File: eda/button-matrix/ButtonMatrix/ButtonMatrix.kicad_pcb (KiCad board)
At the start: 2 copper layers, 191.5 x 87.2 mm, 18 parts, among them SW1 SW_Omron_B3FS, SW10 SW_Omron_B3FS, SW11 SW_Omron_B3FS, SW12 SW_Omron_B3FS, SW13 SW_Omron_B3FS, SW14 SW_Omron_B3FS, SW15 SW_Omron_B3FS, SW16 SW_Omron_B3FS, SW2 SW_Omron_B3FS, SW3 SW_Omron_B3FS, SW4 SW_Omron_B3FS, SW5 SW_Omron_B3FS, SW6 SW_Omron_B3FS, SW7 SW_Omron_B3FS, SW8 SW_Omron_B3FS, SW9 SW_Omron_B3FS

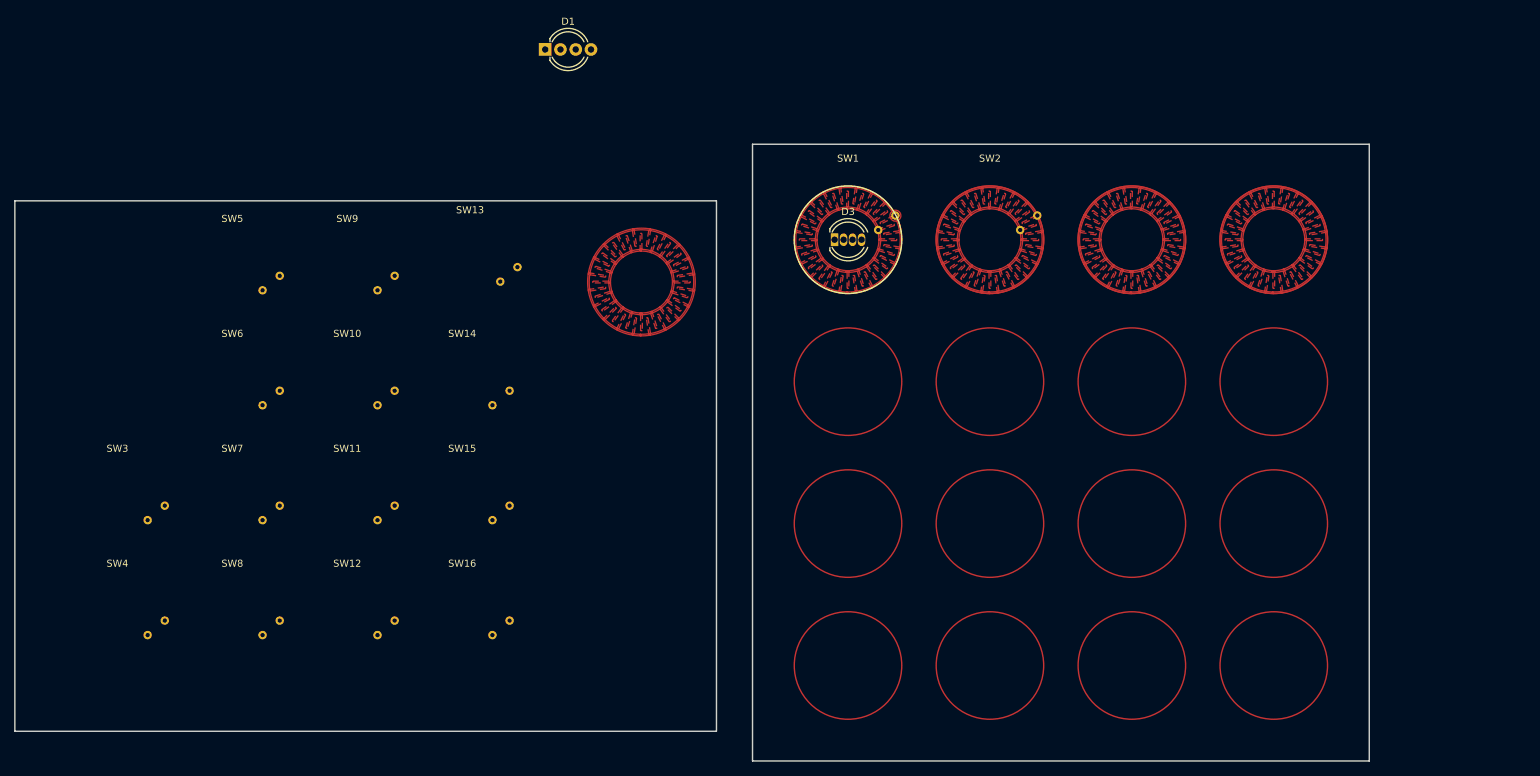
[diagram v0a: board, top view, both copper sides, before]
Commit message: - Updated the pcb for the new 4x4 button matrix - Added support imgui and desktop support
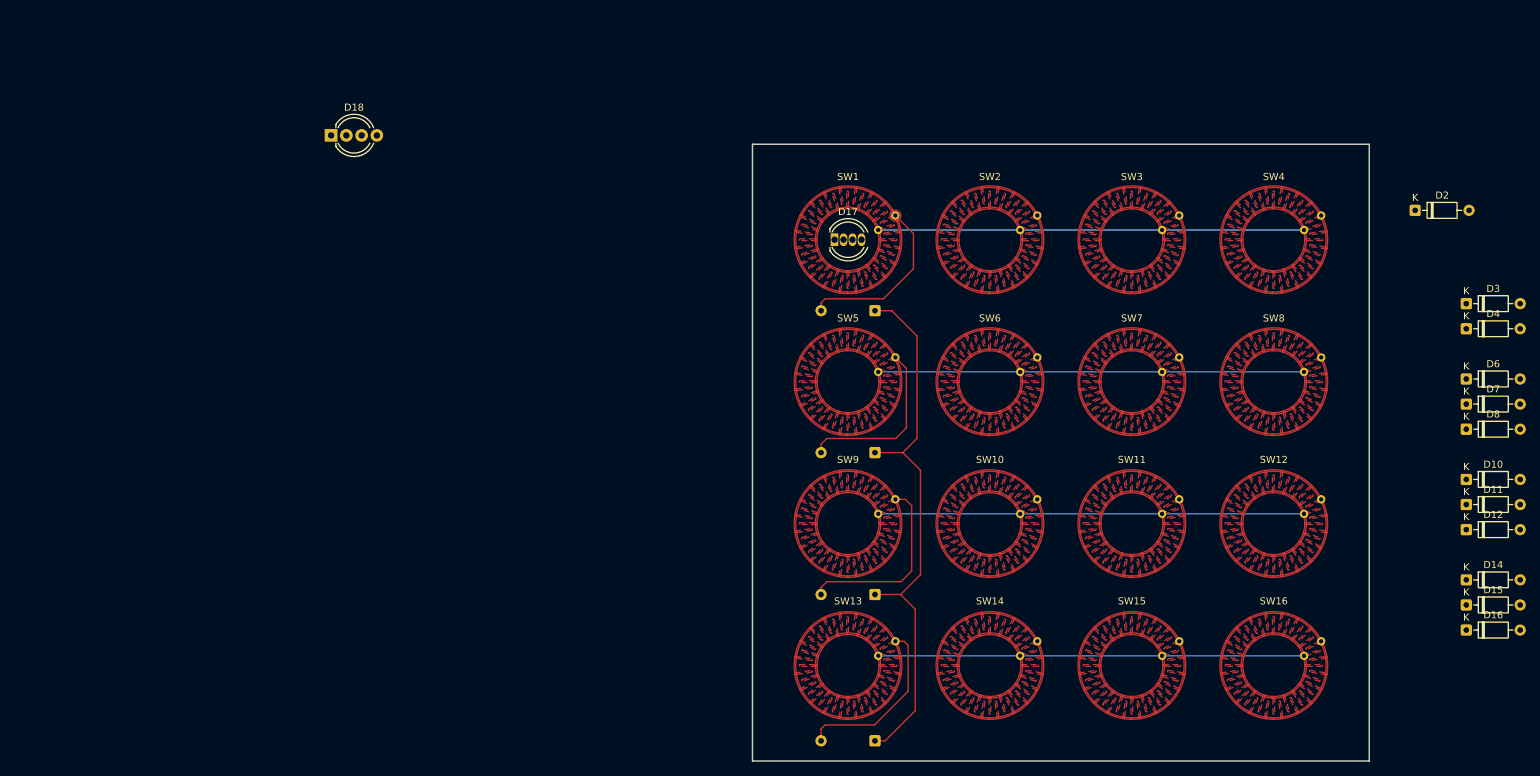
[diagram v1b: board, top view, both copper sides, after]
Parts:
- added D10: 1N4148, Diode_THT:D_DO-35_SOD27_P7.62mm_Horizontal, F.Cu at (228.9, 106.8)
- added D11: 1N4148, Diode_THT:D_DO-35_SOD27_P7.62mm_Horizontal, F.Cu at (228.9, 110.3)
- added D12: 1N4148, Diode_THT:D_DO-35_SOD27_P7.62mm_Horizontal, F.Cu at (228.9, 113.9)
- added D13: 1N4148, Diode_THT:D_DO-35_SOD27_P7.62mm_Horizontal, B.Cu at (145.3, 143.8)
- added D14: 1N4148, Diode_THT:D_DO-35_SOD27_P7.62mm_Horizontal, F.Cu at (228.9, 121.0)
- added D15: 1N4148, Diode_THT:D_DO-35_SOD27_P7.62mm_Horizontal, F.Cu at (228.9, 124.5)
- added D16: 1N4148, Diode_THT:D_DO-35_SOD27_P7.62mm_Horizontal, F.Cu at (228.9, 128.1)
- added D17: LED_RGBA, LED_THT:LED_D5.0mm-4_RGB, F.Cu at (139.6, 72.9)
- added D18: LED_RGBA, LED_THT:LED_D5.0mm-4_RGB_Wide_Pins, F.Cu at (68.4, 58.1)
- added D2: 1N4148, Diode_THT:D_DO-35_SOD27_P7.62mm_Horizontal, F.Cu at (221.7, 68.8)
- added D4: 1N4148, Diode_THT:D_DO-35_SOD27_P7.62mm_Horizontal, F.Cu at (228.9, 85.5)
- added D5: 1N4148, Diode_THT:D_DO-35_SOD27_P7.62mm_Horizontal, B.Cu at (145.3, 103.0)
- added D6: 1N4148, Diode_THT:D_DO-35_SOD27_P7.62mm_Horizontal, F.Cu at (228.9, 92.6)
- added D7: 1N4148, Diode_THT:D_DO-35_SOD27_P7.62mm_Horizontal, F.Cu at (228.9, 96.1)
- added D8: 1N4148, Diode_THT:D_DO-35_SOD27_P7.62mm_Horizontal, F.Cu at (228.9, 99.7)
- added D9: 1N4148, Diode_THT:D_DO-35_SOD27_P7.62mm_Horizontal, B.Cu at (145.3, 123.1)
- D1: value LED_RGBA -> 1N4148; footprint LED_THT:LED_D5.0mm-4_RGB_Wide_Pins -> Diode_THT:D_DO-35_SOD27_P7.62mm_Horizontal; moved to B.Cu
- D3: value LED_RGBA -> 1N4148; footprint LED_THT:LED_D5.0mm-4_RGB -> Diode_THT:D_DO-35_SOD27_P7.62mm_Horizontal
- moved SW4 173.2 mm to (201.7, 72.9)
- moved SW8 151.9 mm to (201.7, 93.0)
- moved SW3 149.2 mm to (181.6, 72.9)
- moved SW12 132.1 mm to (201.7, 113.0)
- moved SW7 128.9 mm to (181.6, 93.0)
- moved SW16 114.8 mm to (201.7, 133.1)
- moved SW11 110.9 mm to (181.6, 113.0)
- moved SW6 107.2 mm to (161.6, 93.0)
- moved SW15 96.6 mm to (181.6, 133.1)
- moved SW10 92.2 mm to (161.6, 113.0)
- moved D3 89.8 mm to (228.9, 81.9)
- moved SW5 87.8 mm to (141.5, 93.0)
- moved SW14 82.6 mm to (161.6, 133.1)
- moved SW9 77.5 mm to (141.5, 113.0)
- moved SW13 75.2 mm to (141.5, 133.1)
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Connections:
- D1 pad 1: unconnected-(D1-RK-Pad1) -> /SW_COL1
- D1 pad 2: unconnected-(D1-GK-Pad2) -> Net-(D1-A)
- D3 pad 1: unconnected-(D3-RK-Pad1) -> /SW_COL3
- D3 pad 2: unconnected-(D3-GK-Pad2) -> Net-(D3-A)
- SW1 pad 1: unconnected-(SW1-Pad1) -> /SW_ROW1
- SW1 pad 2: Net-(SW1-Pad2) -> Net-(D1-A)
- SW10 pad 1: Net-(SW1-Pad2) -> /SW_ROW3
- SW10 pad 2: Net-(SW10-Pad2) -> Net-(D10-A)
- SW11 pad 1: Net-(SW10-Pad2) -> /SW_ROW3
- SW11 pad 2: Net-(SW11-Pad2) -> Net-(D11-A)
- SW12 pad 1: Net-(SW11-Pad2) -> /SW_ROW3
- SW12 pad 2: Net-(SW12-Pad2) -> Net-(D12-A)
- SW13 pad 1: unconnected-(SW13-Pad1) -> /SW_ROW4
- SW13 pad 2: Net-(SW1-Pad2) -> Net-(D13-A)
- SW14 pad 1: Net-(SW1-Pad2) -> /SW_ROW4
- SW14 pad 2: Net-(SW10-Pad2) -> Net-(D14-A)
- SW15 pad 1: Net-(SW10-Pad2) -> /SW_ROW4
- SW15 pad 2: Net-(SW11-Pad2) -> Net-(D15-A)
- SW16 pad 1: Net-(SW11-Pad2) -> /SW_ROW4
- SW16 pad 2: Net-(SW12-Pad2) -> Net-(D16-A)
- SW2 pad 1: Net-(SW1-Pad2) -> /SW_ROW1
- SW2 pad 2: Net-(SW10-Pad2) -> Net-(D2-A)
- SW3 pad 1: Net-(SW10-Pad2) -> /SW_ROW1
- SW3 pad 2: Net-(SW11-Pad2) -> Net-(D3-A)
- SW4 pad 1: Net-(SW11-Pad2) -> /SW_ROW1
- SW4 pad 2: Net-(SW12-Pad2) -> Net-(D4-A)
- SW5 pad 1: unconnected-(SW5-Pad1) -> /SW_ROW2
- SW5 pad 2: Net-(SW1-Pad2) -> Net-(D5-A)
- SW6 pad 1: Net-(SW1-Pad2) -> /SW_ROW2
- SW6 pad 2: Net-(SW10-Pad2) -> Net-(D6-A)
- SW7 pad 1: Net-(SW10-Pad2) -> /SW_ROW2
- SW7 pad 2: Net-(SW11-Pad2) -> Net-(D7-A)
- SW8 pad 1: Net-(SW11-Pad2) -> /SW_ROW2
- SW8 pad 2: Net-(SW12-Pad2) -> Net-(D8-A)
- SW9 pad 1: unconnected-(SW9-Pad1) -> /SW_ROW3
- SW9 pad 2: Net-(SW1-Pad2) -> Net-(D9-A)
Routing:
- net /SW_COL1: track 0.00 -> 79.3 mm
- net /SW_ROW4: track 0.00 -> 60.2 mm
- net /SW_ROW3: track 0.00 -> 60.2 mm
- net /SW_ROW2: track 0.00 -> 60.2 mm
- net /SW_ROW1: track 0.00 -> 60.2 mm
- net Net-(D9-A): track 0.00 -> 26.7 mm
- net Net-(D5-A): track 0.00 -> 24.8 mm
- net Net-(D1-A): track 0.00 -> 24.8 mm
- net Net-(D13-A): track 0.00 -> 24.7 mm
- added copper zone on F.Cu, net /SW_ROW1
- added copper zone on F.Cu, net /SW_ROW2
- added copper zone on F.Cu, net /SW_ROW3
- added copper zone on F.Cu, net /SW_ROW4
- added copper zone on F.Cu, net Net-(D1-A)
- added copper zone on F.Cu, net Net-(D10-A)
- added copper zone on F.Cu, net Net-(D11-A)
- added copper zone on F.Cu, net Net-(D12-A)
- added copper zone on F.Cu, net Net-(D13-A)
- added copper zone on F.Cu, net Net-(D14-A)
- added copper zone on F.Cu, net Net-(D15-A)
- added copper zone on F.Cu, net Net-(D16-A)
- added copper zone on F.Cu, net Net-(D2-A)
- added copper zone on F.Cu, net Net-(D3-A)
- added copper zone on F.Cu, net Net-(D4-A)
- added copper zone on F.Cu, net Net-(D5-A)
- added copper zone on F.Cu, net Net-(D6-A)
- added copper zone on F.Cu, net Net-(D7-A)
- added copper zone on F.Cu, net Net-(D8-A)
- added copper zone on F.Cu, net Net-(D9-A)
- removed copper zone on F.Cu, net Net-(SW1-Pad2)
- removed copper zone on F.Cu, net unconnected-(SW13-Pad1)
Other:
- board size 191.5 x 87.2 mm -> 87.2 x 87.2 mm

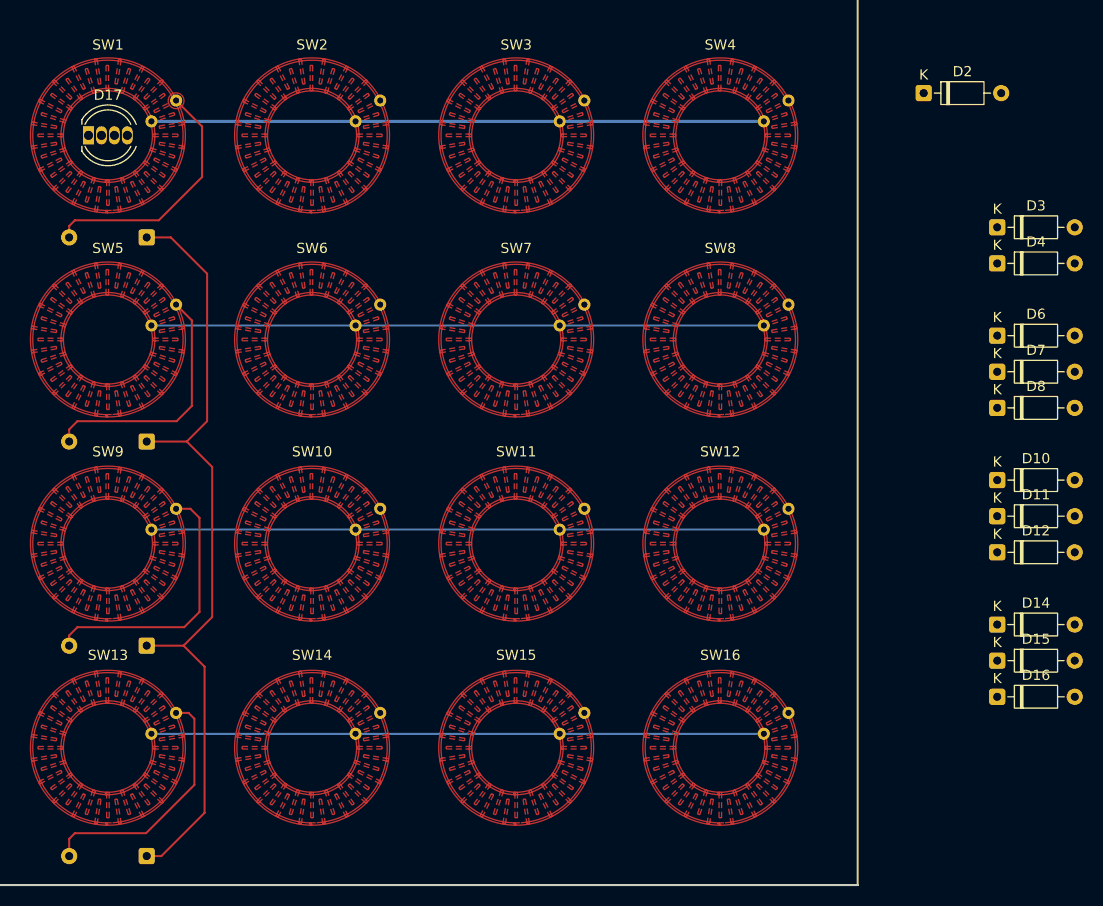
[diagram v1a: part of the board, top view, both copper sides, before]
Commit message: - Updates to button matrix pcb
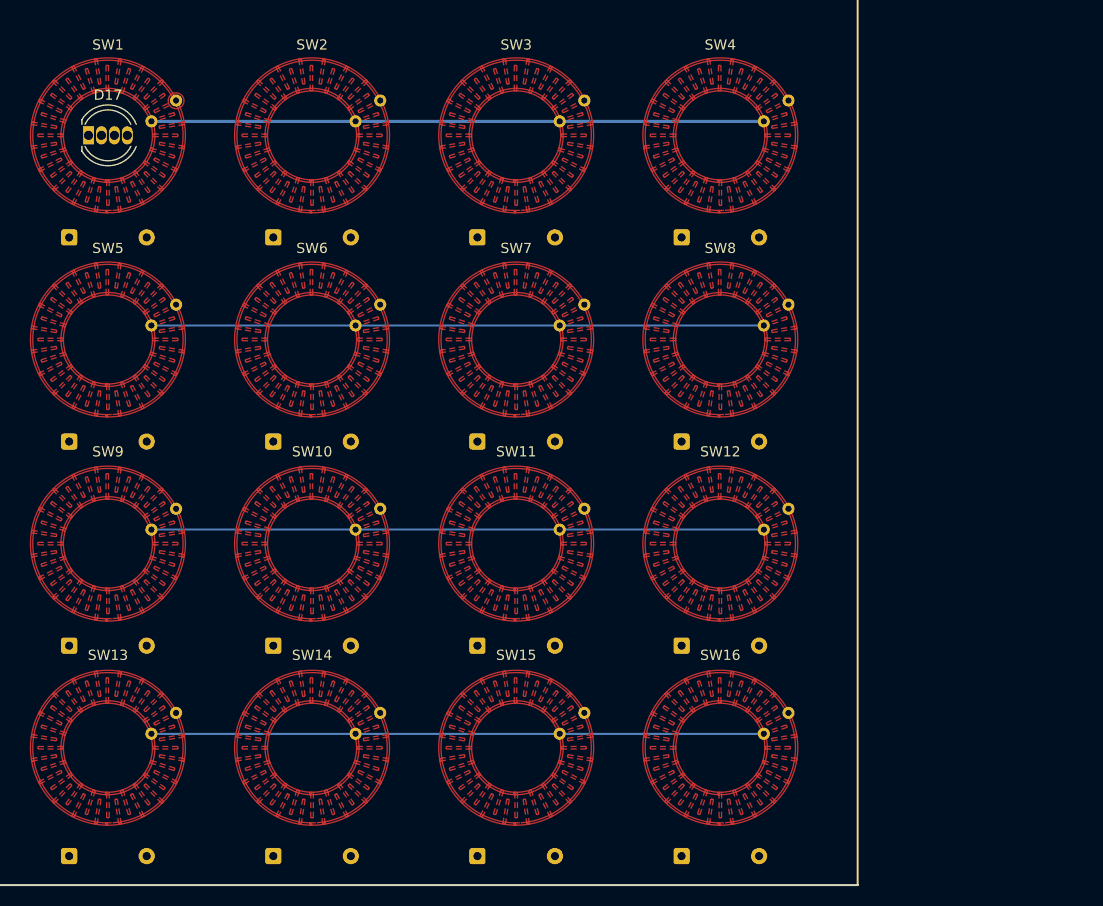
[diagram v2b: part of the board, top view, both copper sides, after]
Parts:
- D10, D11, D12, D14, D15, D16, D2, D3, D4, D6, D7, D8: moved to B.Cu
- moved D14 74.7 mm to (157.8, 143.8)
- moved D10 73.0 mm to (157.8, 123.1)
- moved D6 71.9 mm to (157.8, 103.0)
- moved D2 65.5 mm to (157.8, 82.9)
- moved D15 54.6 mm to (177.8, 143.8)
- moved D11 52.7 mm to (177.8, 123.1)
- moved D7 51.6 mm to (177.8, 103.0)
- moved D3 51.1 mm to (177.8, 82.9)
- moved D16 34.8 mm to (197.9, 143.8)
- moved D12 32.4 mm to (197.9, 123.1)
- moved D8 31.2 mm to (197.9, 103.0)
- moved D4 31.1 mm to (197.9, 82.9)
- moved D1 7.62 mm to (137.7, 82.9), turned to 0 degrees
- moved D13 7.62 mm to (137.7, 143.8), turned to 0 degrees
- moved D5 7.62 mm to (137.7, 103.0), turned to 0 degrees
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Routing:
- net /SW_COL1: track 79.3 -> 0.00 mm
- net Net-(D9-A): track 26.7 -> 0.00 mm
- net Net-(D5-A): track 24.8 -> 0.00 mm
- net Net-(D1-A): track 24.8 -> 0.00 mm
- net Net-(D13-A): track 24.7 -> 0.00 mm
